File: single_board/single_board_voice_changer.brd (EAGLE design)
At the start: 58.1 x 58.4 mm, 24 parts, among them IC2 MCP3202P, U1 ATMEGA328P_PDIP

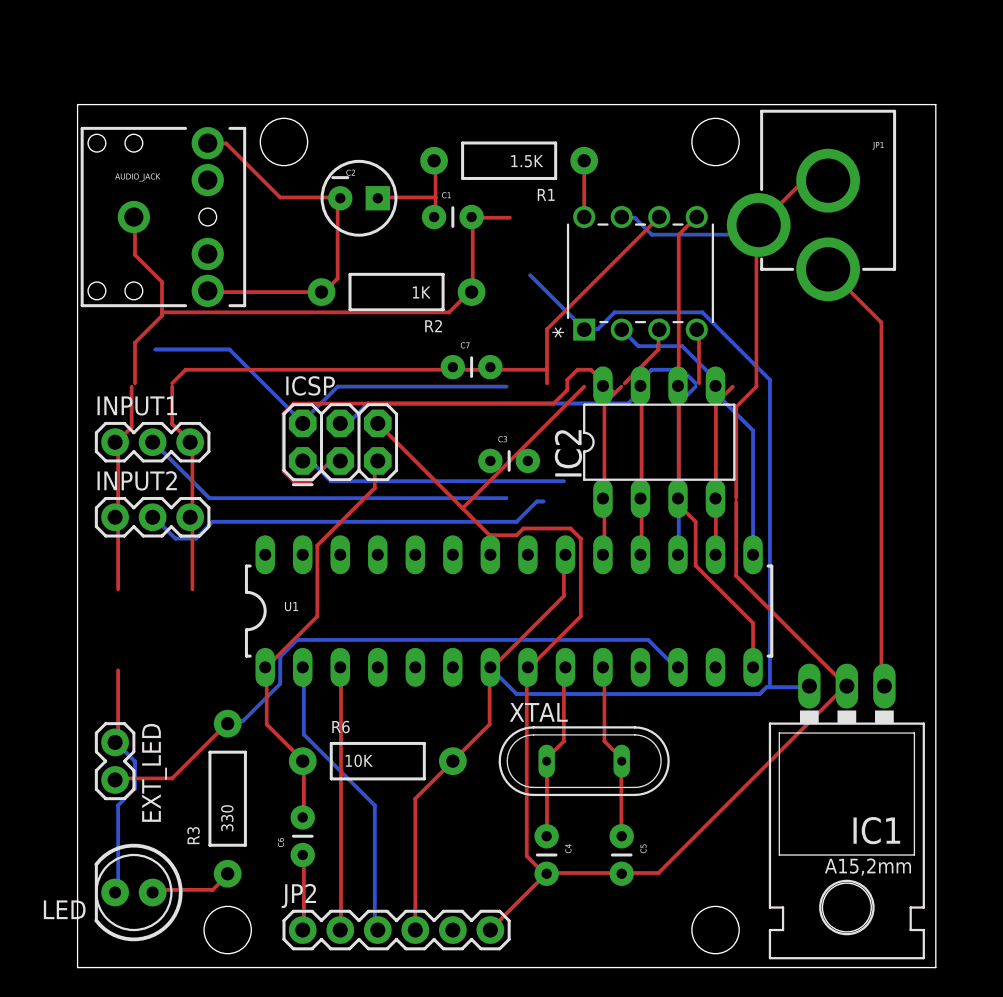
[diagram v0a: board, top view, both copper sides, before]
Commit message: redo board
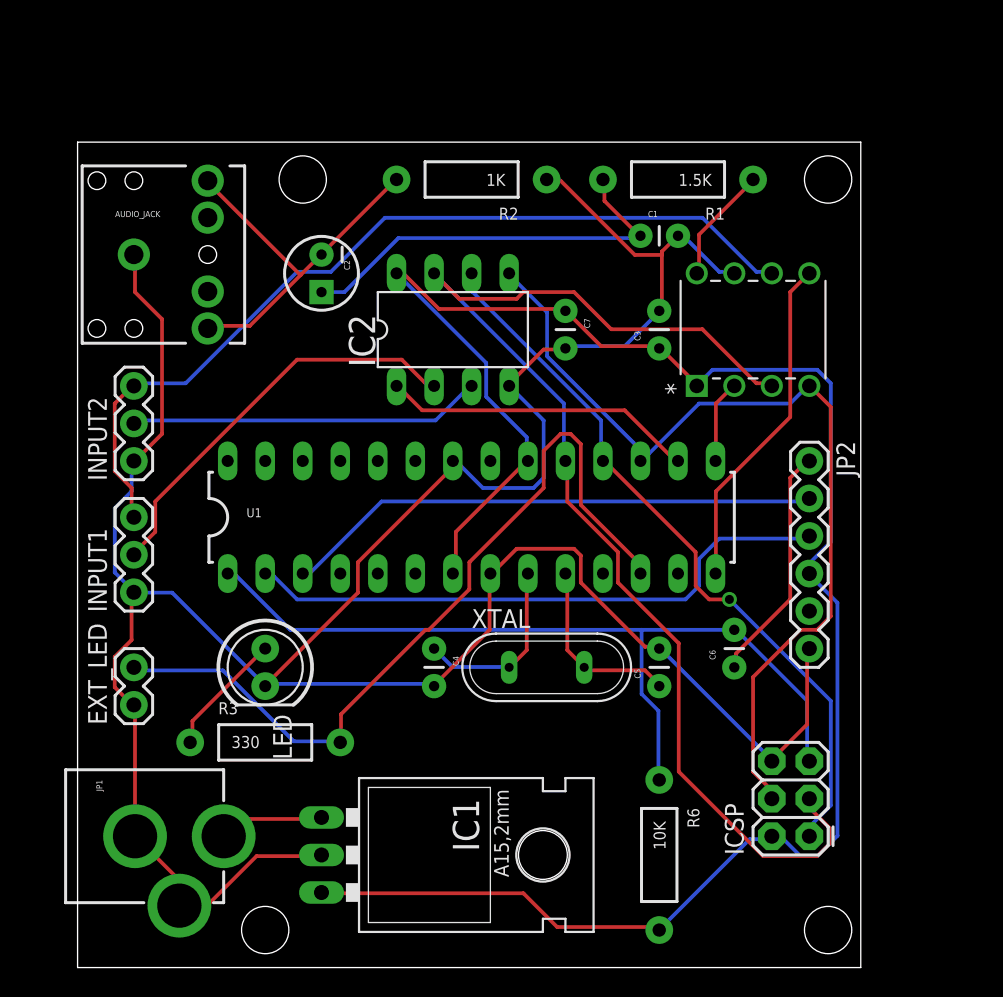
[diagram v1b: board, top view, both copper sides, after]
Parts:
- moved JP1 75.5 mm to (-3.81, 8.89), turned to 270 degrees
- moved JP2 46.7 mm to (49.5, 34.3), turned to 270 degrees
- moved ICSP 42.7 mm to (49.5, 8.89), turned to 90 degrees
- moved IC1 32.7 mm to (20.3, 7.62), turned to 270 degrees
- moved C6 31.9 mm to (44.5, 20.3)
- moved R6 20.1 mm to (39.4, 7.62), turned to 270 degrees
- moved LED 17.6 mm to (12.7, 20.3), turned to 270 degrees
- moved IC2 15.9 mm to (25.4, 43.2)
- moved C4 14.8 mm to (24.1, 21.6)
- moved C1 14.0 mm to (38.1, 49.5)
- moved C3 13.7 mm to (39.4, 41.9), turned to 90 degrees
- moved R1 11.5 mm to (40.6, 53.3)
- moved C5 10.5 mm to (39.4, 19.1), turned to 90 degrees
- moved INPUT1 10.2 mm to (3.81, 25.4), turned to 90 degrees
- moved R2 9.16 mm to (26.7, 53.3)
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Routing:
- net SCK: track 49.7 -> 83.8 mm
- net RESET: track 28.5 -> 57.6 mm
- net N$4: track 29.8 -> 7.16 mm
- net MISO: track 28.5 -> 49.7 mm, vias 0 -> 1
- net RX: track 19.9 -> 40.4 mm
- net MOSI: track 42.0 -> 62.5 mm
- net N$2: track 7.80 -> 28.1 mm
- net TX: track 17.8 -> 36.4 mm
- net SS_DAC: track 20.7 -> 5.64 mm
- net GND: track 209.7 -> 195.8 mm
- net VCC: track 119.9 -> 131.6 mm
- net LED: track 43.8 -> 55.4 mm
- net DTR: track 5.13 -> 16.2 mm
- net LDAC: track 33.1 -> 23.0 mm
- net SS_ADC: track 11.9 -> 21.1 mm
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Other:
- board size 58.1 x 58.4 mm -> 53 x 55.9 mm

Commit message: another rev of the board design
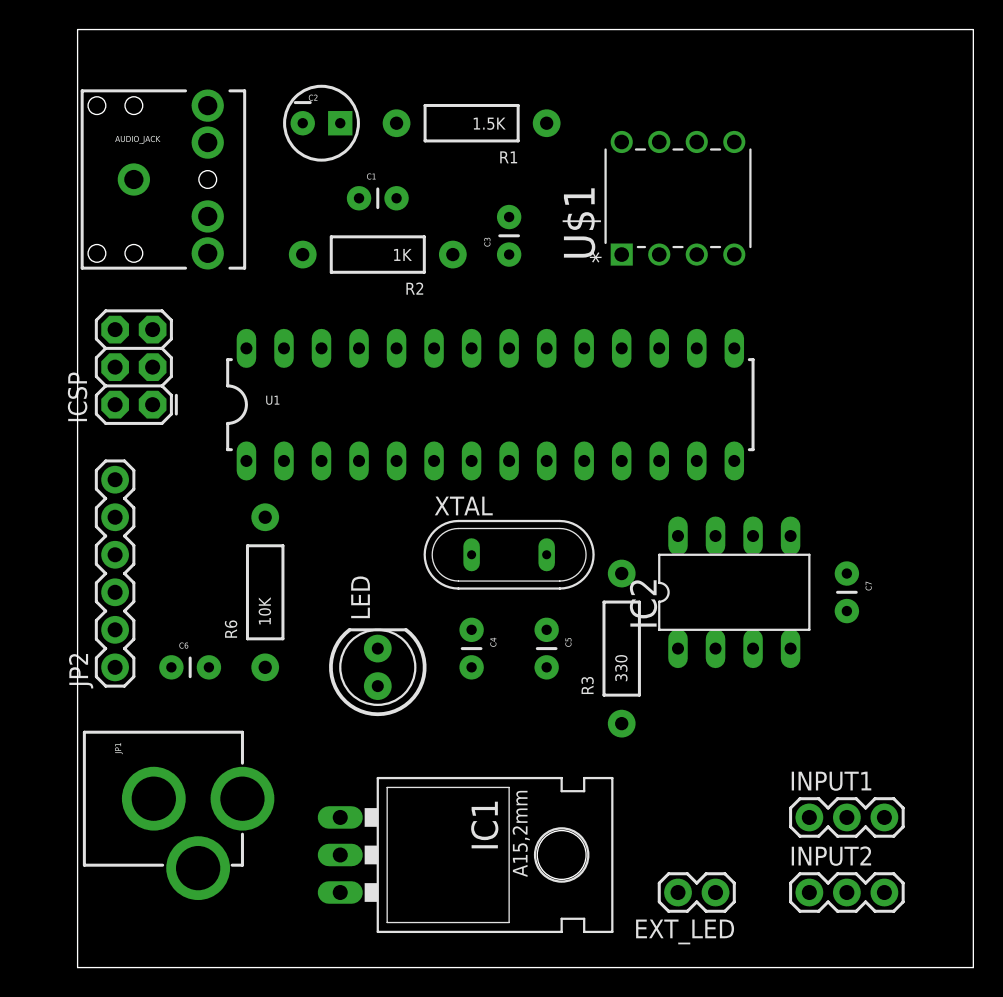
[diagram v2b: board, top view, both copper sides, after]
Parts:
- moved INPUT2 54.3 mm to (49.5, 5.08), turned to 0 degrees
- moved ICSP 53.2 mm to (5.08, 38.1)
- moved JP2 49.0 mm to (2.54, 20.3), turned to 90 degrees
- moved INPUT1 48.2 mm to (49.5, 10.2), turned to 0 degrees
- moved EXT_LED 41.4 mm to (43.2, 5.08), turned to 180 degrees
- moved C6 38.1 mm to (6.35, 20.3), turned to 0 degrees
- moved R6 32.1 mm to (12.7, 25.4), turned to 90 degrees
- moved IC2 26.1 mm to (44.5, 25.4)
- moved C7 26.1 mm to (52.1, 26.7)
- moved R3 25.0 mm to (36.8, 21.6), turned to 90 degrees
- moved C1 19.2 mm to (19.1, 52.1)
- moved R1 14.5 mm to (26.7, 57.1)
- moved C3 12.0 mm to (29.2, 48.3)
- moved U$1 10.2 mm to (44.5, 55.9)
- moved C2 10.2 mm to (16.5, 57.1), turned to 0 degrees
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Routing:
- net GND: track 195.8 -> 0.00 mm
- net VCC: track 131.6 -> 0.00 mm
- net SCK: track 83.8 -> 0.00 mm
- net MOSI: track 62.5 -> 0.00 mm
- net VREF: track 59.5 -> 0.00 mm
- net RESET: track 57.6 -> 0.00 mm
- net LED: track 55.4 -> 0.00 mm
- net MISO: track 49.7 -> 0.00 mm, vias 1 -> 0
- net RX: track 40.4 -> 0.00 mm
- net TX: track 36.4 -> 0.00 mm
- net N$2: track 28.1 -> 0.00 mm
- net ADC_CH0: track 27.8 -> 0.00 mm
- net N$10: track 26.0 -> 0.00 mm
- net ADC_CH1: track 24.0 -> 0.00 mm
- net LDAC: track 23.0 -> 0.00 mm
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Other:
- board size 53 x 55.9 mm -> 60.6 x 63.5 mm

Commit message: another rev of the board design
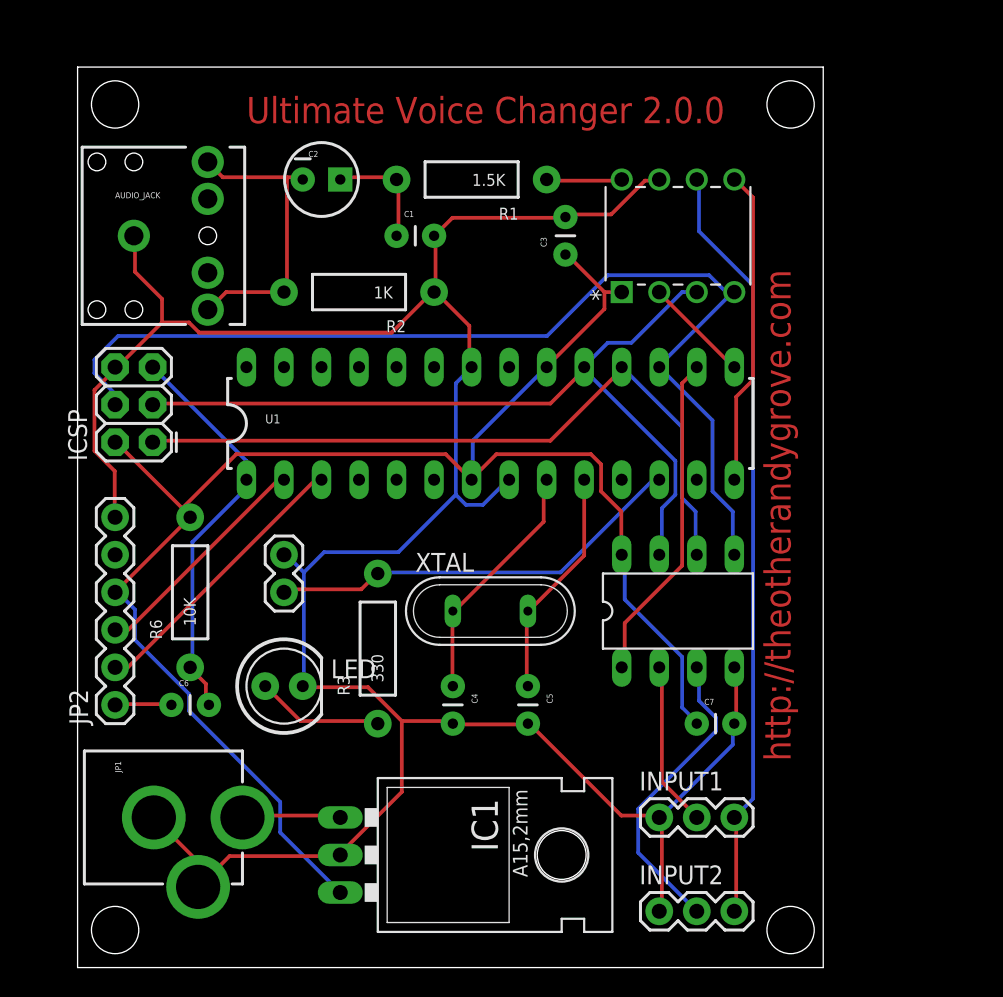
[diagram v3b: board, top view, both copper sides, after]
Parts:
- moved EXT_LED 37.1 mm to (14.0, 27.9), turned to 270 degrees
- moved R3 16.5 mm to (20.3, 21.6)
- moved C7 14.4 mm to (41.9, 16.5), turned to 0 degrees
- moved INPUT2 10.2 mm to (39.4, 3.81)
- moved INPUT1 10.2 mm to (39.4, 10.2)
- moved LED 6.48 mm to (14.0, 19.1), turned to 0 degrees
- moved R6 5.08 mm to (7.62, 25.4)
- moved IC2 4.02 mm to (40.6, 24.1)
- moved XTAL 4.02 mm to (27.9, 24.1)
- moved C4 4.02 mm to (25.4, 19.1)
- moved C5 4.02 mm to (30.5, 19.1)
- moved AUDIO_JACK 3.81 mm to (3.81, 49.5)
- moved C3 3.81 mm to (33.0, 48.3)
- moved C2 3.81 mm to (16.5, 53.3)
- moved R1 3.81 mm to (26.7, 53.3)
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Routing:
- net GND: track 0.00 -> 179.8 mm
- net VCC: track 0.00 -> 115.1 mm
- net MOSI: track 0.00 -> 72.0 mm
- net SCK: track 0.00 -> 55.8 mm
- net VREF: track 0.00 -> 51.8 mm
- net MISO: track 0.00 -> 48.7 mm
- net LED: track 0.00 -> 28.6 mm
- net RESET: track 0.00 -> 27.7 mm
- net SS_ADC: track 0.00 -> 22.5 mm
- net LDAC: track 0.00 -> 21.4 mm
- net ADC_CH1: track 0.00 -> 20.9 mm
- net N$10: track 0.00 -> 20.5 mm
- net TX: track 0.00 -> 19.2 mm
- net N$5: track 0.00 -> 16.7 mm
- net RX: track 0.00 -> 15.7 mm
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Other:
- board size 60.6 x 63.5 mm -> 50.5 x 61 mm
- board text added: "Ultimate Voice Changer 2.0.0"
- board text added: "http://theotherandygrove.com"
